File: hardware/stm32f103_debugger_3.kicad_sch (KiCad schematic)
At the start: 18 parts, among them J1 GMSB0531112YEU, J2 Conn_01x06, SW1 SW TACT-SPST, U1 STM32F103CBT6, Y1 ABM8G-8.000MHZ-18-D2Y-T

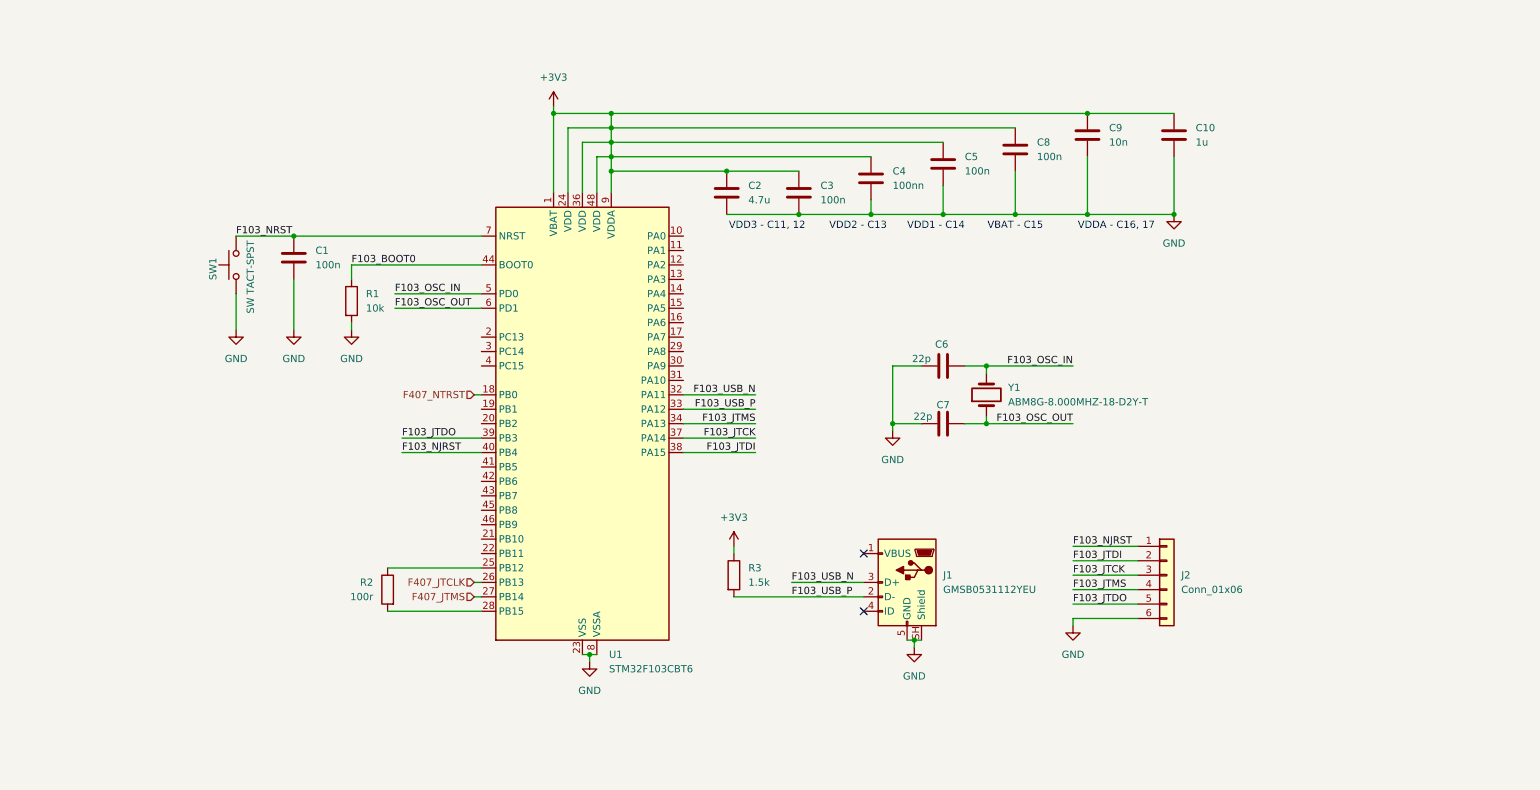
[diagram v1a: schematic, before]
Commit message: Organize schematic
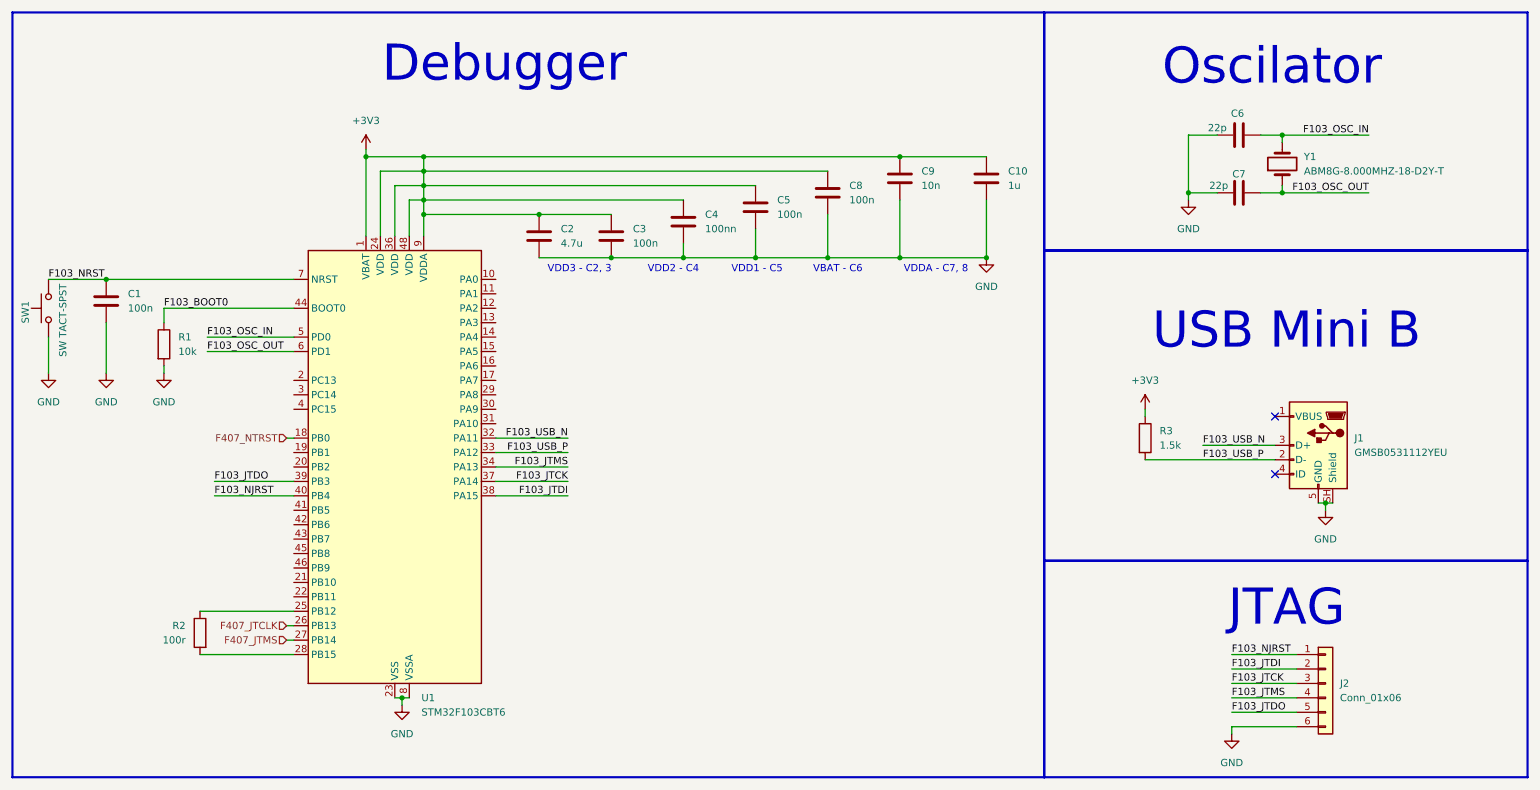
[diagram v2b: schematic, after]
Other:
- note added: "Debugger"
- note added: "JTAG"
- note added: "Oscilator"
- note added: "USB Mini B"
- note added: "VBAT - C6"
- note added: "VDD1 - C5"
- note added: "VDD2 - C4"
- note added: "VDD3 - C2, 3"
- note added: "VDDA - C7, 8"
- note removed: "VBAT - C15"
- note removed: "VDD1 - C14"
- note removed: "VDD2 - C13"
- note removed: "VDD3 - C11, 12"
- note removed: "VDDA - C16, 17"
- moved on the sheet: C1, C10, C2, C3, C4, C5, C6, C7, C8, C9, J1, J2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
